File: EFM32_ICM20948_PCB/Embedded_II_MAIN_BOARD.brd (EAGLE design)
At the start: 52.8 x 35.1 mm, 98 parts, among them IC2 EFM32HG322F64G-C-QFP48R, IC5 TPS7A0518PDBZR, Q1 20V/0.2A/8MHz/1.2Ω/1Vth, Q6 20V/0.2A/8MHz/1.2Ω/1Vth, Q8 20V/0.2A/8MHz/1.2Ω/1Vth, U3 9DoF IMU, Y2 FC-135_32.7680KA-A3, Y3 ABM3B-24.000MHZ-B2-T

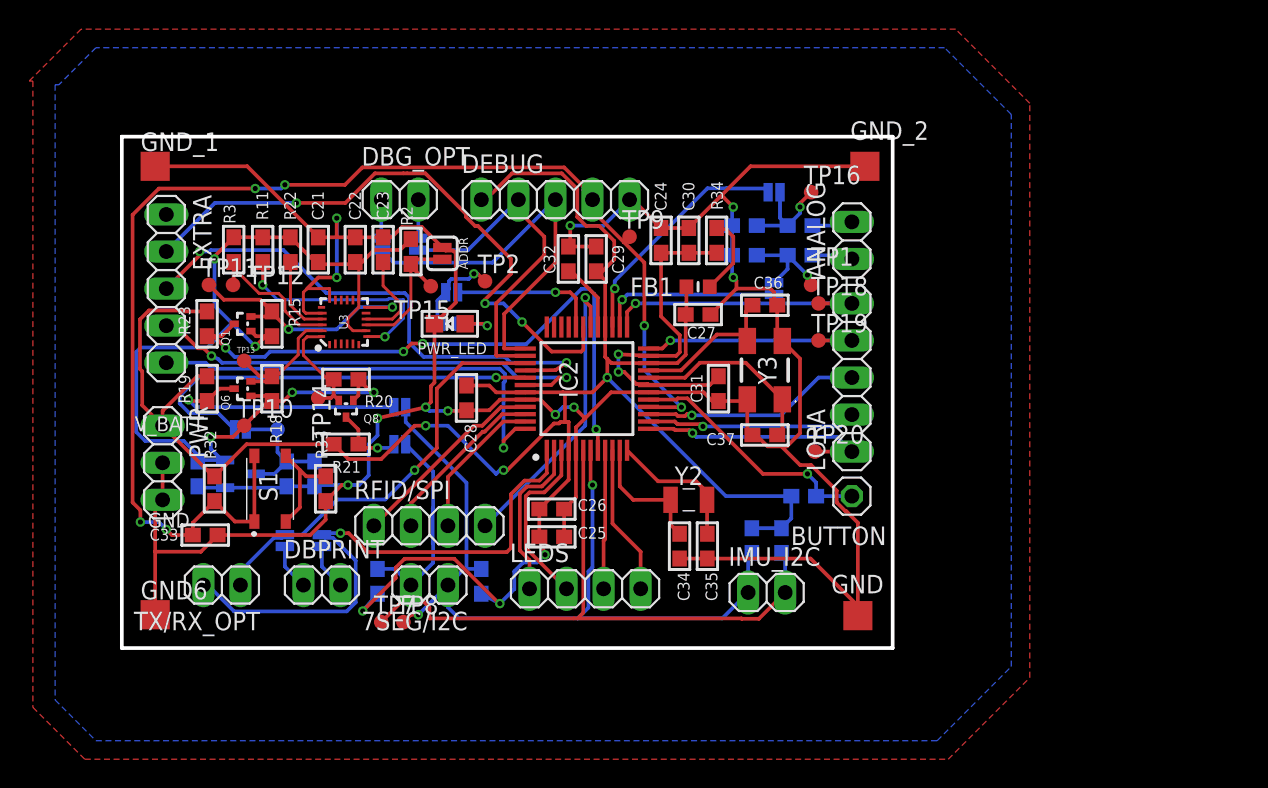
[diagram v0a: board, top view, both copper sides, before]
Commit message: main pcb lora update, bijna klaar
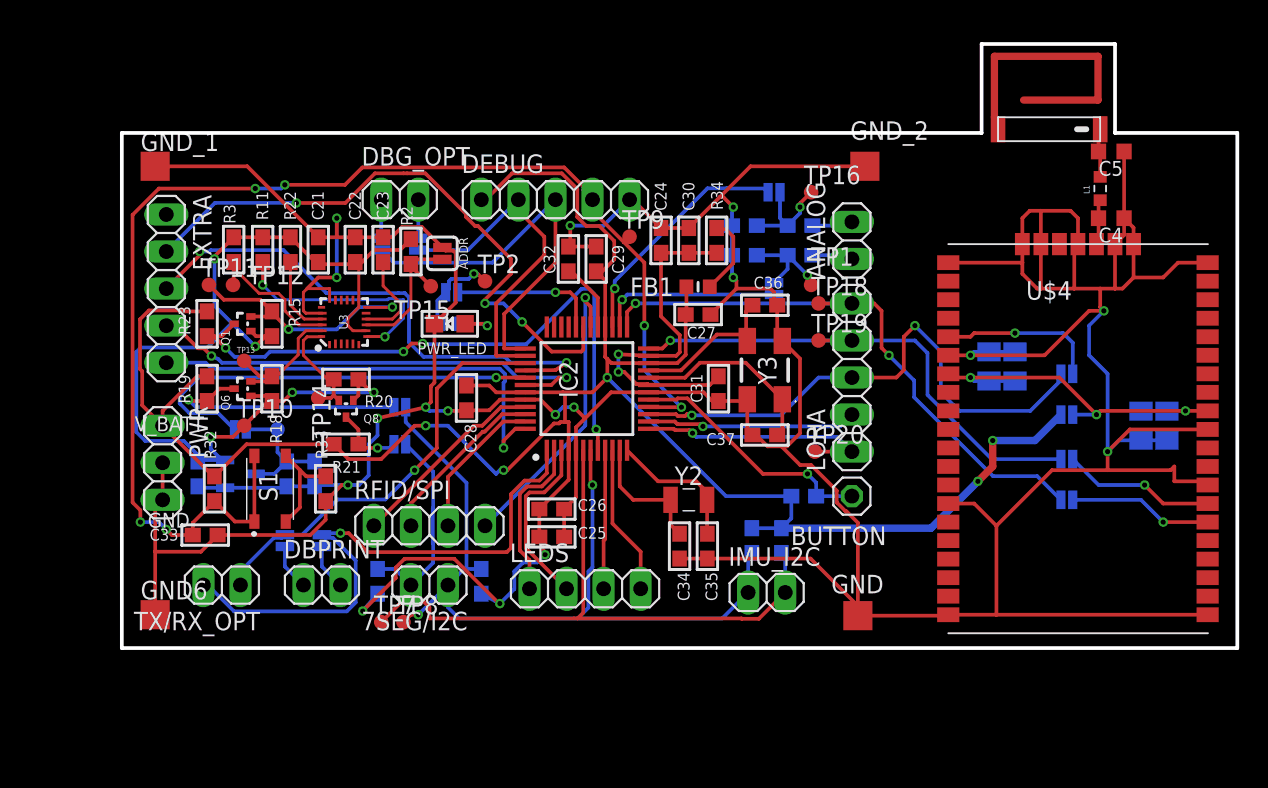
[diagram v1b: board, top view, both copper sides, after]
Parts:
- added C2, C6: 10u, rcl:C0805K
- added C3, C7: 100n, rcl:C0805K
- added C4, C5: (no value), rcl:C0603K
- added L1: WE-MK_0603_744786118, project:WE-MK_0603
- added LORA_RESET: LORA_RESET, SparkFun-Jumpers:SMT-JUMPER_2_NO_SILK
- added LORA_RX: LORA_RX, SparkFun-Jumpers:SMT-JUMPER_2_NO_SILK
- added LORA_TX: LORA_TX, SparkFun-Jumpers:SMT-JUMPER_2_NO_SILK
- added LORA_VDD: LORA_VDD, SparkFun-Jumpers:SMT-JUMPER_2_NO_SILK
- added U$2: ANTENNA868, project:CERAMIC-ANTENNA
- added U$4: RN2483, project:RN2483
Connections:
- new net N$1: C5.2, L1.2, U$2.P$1
- new net N$2: C4.2, L1.1, U$4.RFH
- new net N$6: LORA_RX.2, U$4.UART_RX
- new net N$7: LORA_TX.2, U$4.UART_TX
- new net N$8: LORA_RESET.2, U$4.RESET°
- new net VDD_LORA: C2.1, C3.1, C6.1, C7.1, LORA_VDD.2, U$4.VDD, U$4.VDD2
- net GND: now also C2.2, C3.2, C4.1, C5.1, C6.2, C7.2, U$4.GND, U$4.GND1, U$4.GND10, U$4.GND11, U$4.GND12, U$4.GND2, U$4.GND3, U$4.GND4, U$4.GND5, U$4.GND6, U$4.GND7, U$4.GND8, U$4.GND9
- net LORA_!RESET!: now also LORA_RESET.1
- net LORA_RX: now also LORA_RX.1
- net LORA_TX: now also LORA_TX.1
- net VDD: now also LORA_VDD.1
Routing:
- net GND: track 211.8 -> 354.8 mm, vias 11 -> 14
- net VDD_LORA: track 0.00 -> 26.9 mm, vias 0 -> 3
- net VDD: track 149.5 -> 172.9 mm, vias 6 -> 8
- net LORA_!RESET!: track 15.1 -> 37.6 mm, vias 1 -> 2
- net LORA_TX: track 19.0 -> 41.0 mm, vias 1 -> 2
- net LORA_RX: track 16.5 -> 35.8 mm
- net N$8: track 0.00 -> 11.0 mm, vias 0 -> 1
- net N$6: track 0.00 -> 10.5 mm, vias 0 -> 1
- net N$7: track 0.00 -> 9.88 mm, vias 0 -> 1
- net N$1: track 0.00 -> 3.36 mm
- net N$2: track 0.00 -> 3.12 mm
- removed copper zone on layer 1, net GND
- removed copper zone on layer 16, net GND
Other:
- board size 52.8 x 35.1 mm -> 76.5 x 41.4 mm
